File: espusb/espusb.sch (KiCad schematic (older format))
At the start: 10 parts, among them P1 USB_A, U1 MCP1603, U2 FT232

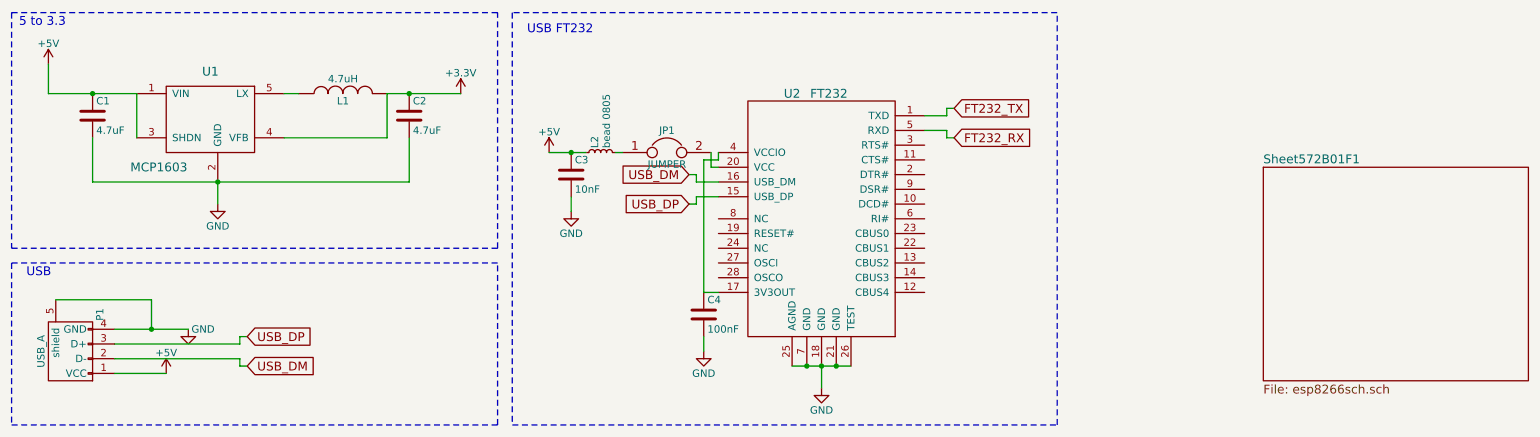
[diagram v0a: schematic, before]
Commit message: r6 version (with ch340)
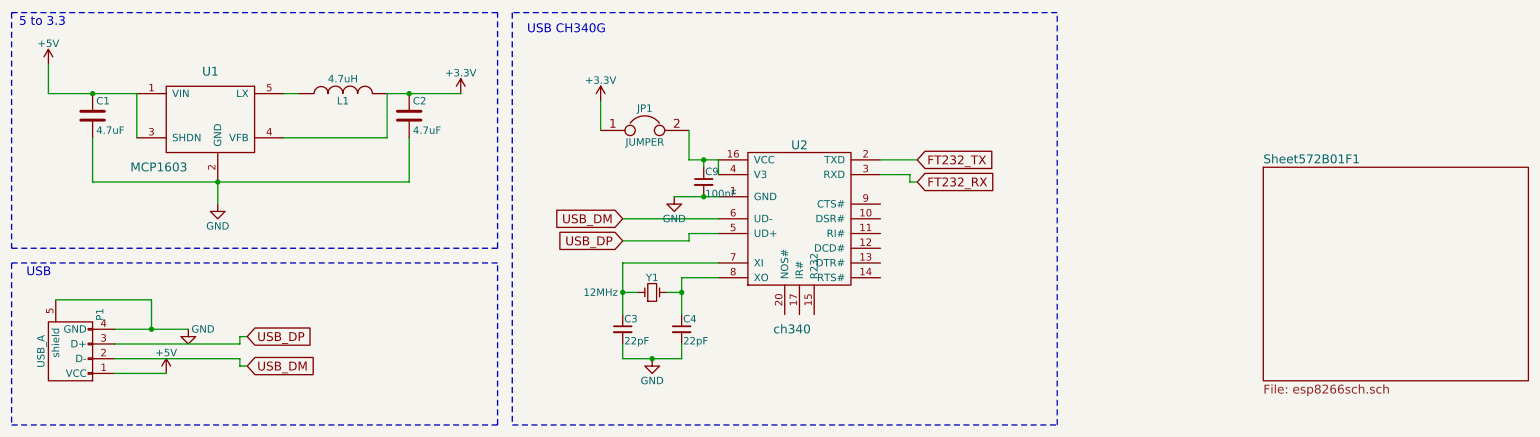
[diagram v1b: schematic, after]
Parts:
- removed C3: 10nF, Resistors_SMD:R_0603_HandSoldering, symbol C
- removed C4: 100nF, Resistors_SMD:R_0603_HandSoldering, symbol C
- removed L2: bead 0805, Resistors_SMD:R_0805_HandSoldering, symbol L_Small
- removed U2: FT232, espusb:SSOP-28_5.3x10.2mm_Pitch0.65mm, symbol FT232
- added C3, C4: 22pF, Capacitors_SMD:C_0603, symbol C_Small
- added C9: 100nF, Capacitors_SMD:C_0805, symbol C_Small
- added U2: ch340, SMD_Packages:SO-16-N, symbol ch340
- added Y1: 12MHz, Crystals:HC-49V, symbol Crystal_Small
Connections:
- net +3V3: now also JP1.1
- net FT232_RX: now also U2.3 (RXD)
- net FT232_TX: now also U2.2 (TXD)
- net GND: now also C3.2, C4.2, C9.2, U2.1 (GND)
- net USB_DM: now also U2.6 (UD-)
- net USB_DP: now also U2.5 (UD+)
- net at JP1.2: now also C9.1, U2.16 (VCC), U2.4 (V3)
- new net: C3.1, U2.7 (XI), Y1.1
- new net: C4.1, U2.8 (XO), Y1.2
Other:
- note added: "USB CH340G"
- note removed: "USB FT232"
- moved on the sheet: JP1
